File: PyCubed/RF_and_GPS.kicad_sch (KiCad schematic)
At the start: 45 parts, among them IC2 PCF8523T_1,118, J11 73412-0114, J12 73412-0114, J7 73412-0114, Q17 BSS138DWQ-7, Q28 MBT2222ADW1T1, Q29 BSS138DWQ-7, Q30 MBT2222ADW1T1, U10 XTB-40, U12 XTB-40, U13 EP2W+, U14 S1216V8, U20 RFM9xBreakout, U23 RFM98PW

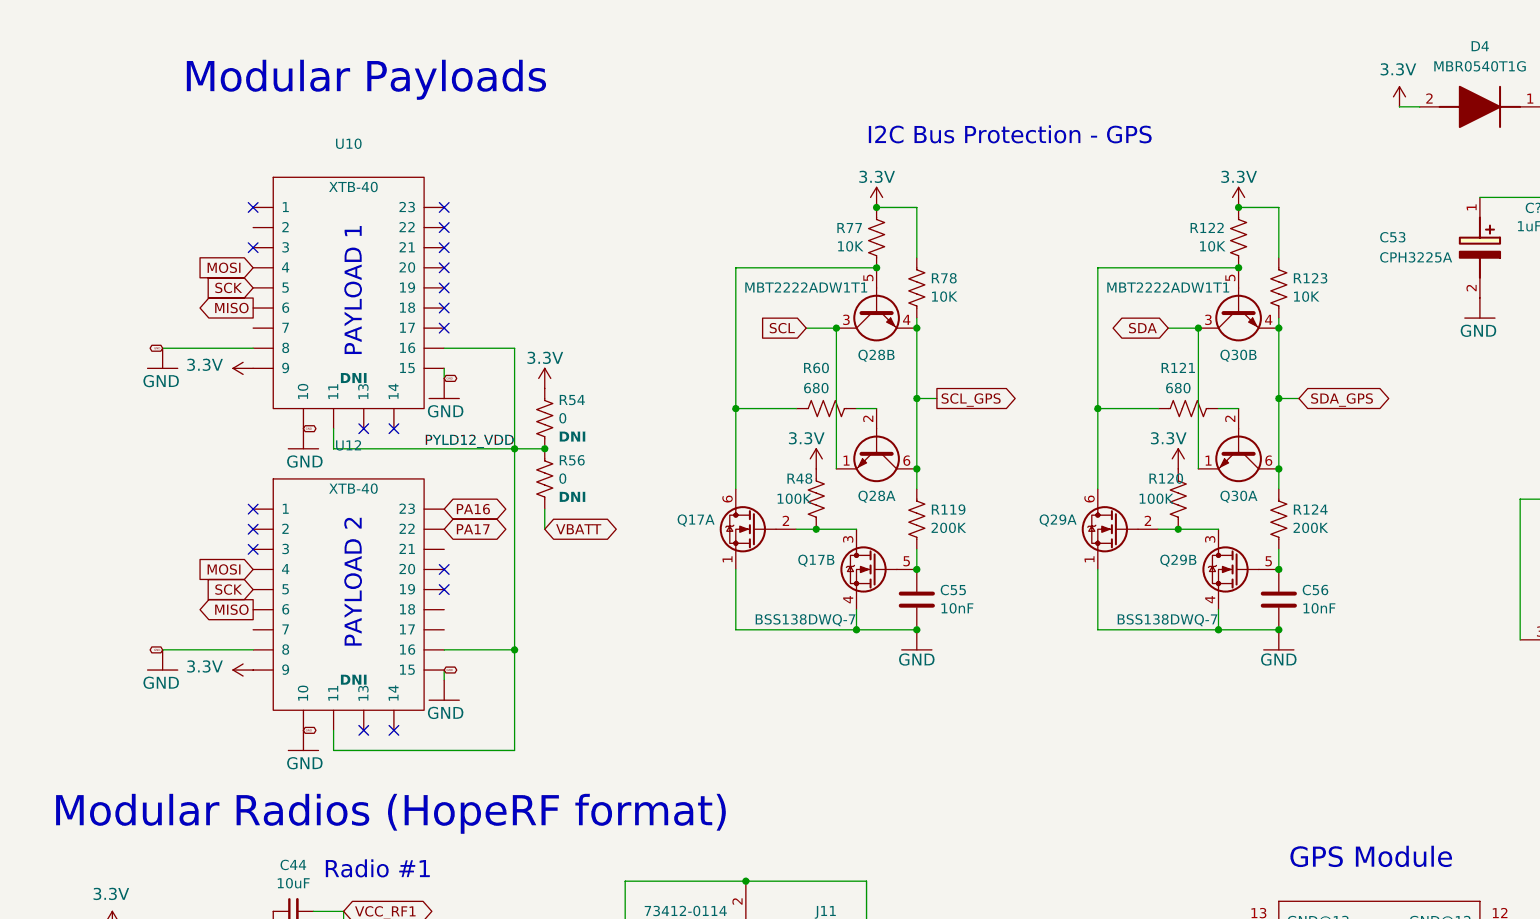
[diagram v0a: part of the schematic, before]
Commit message: PyCubed Routing Done
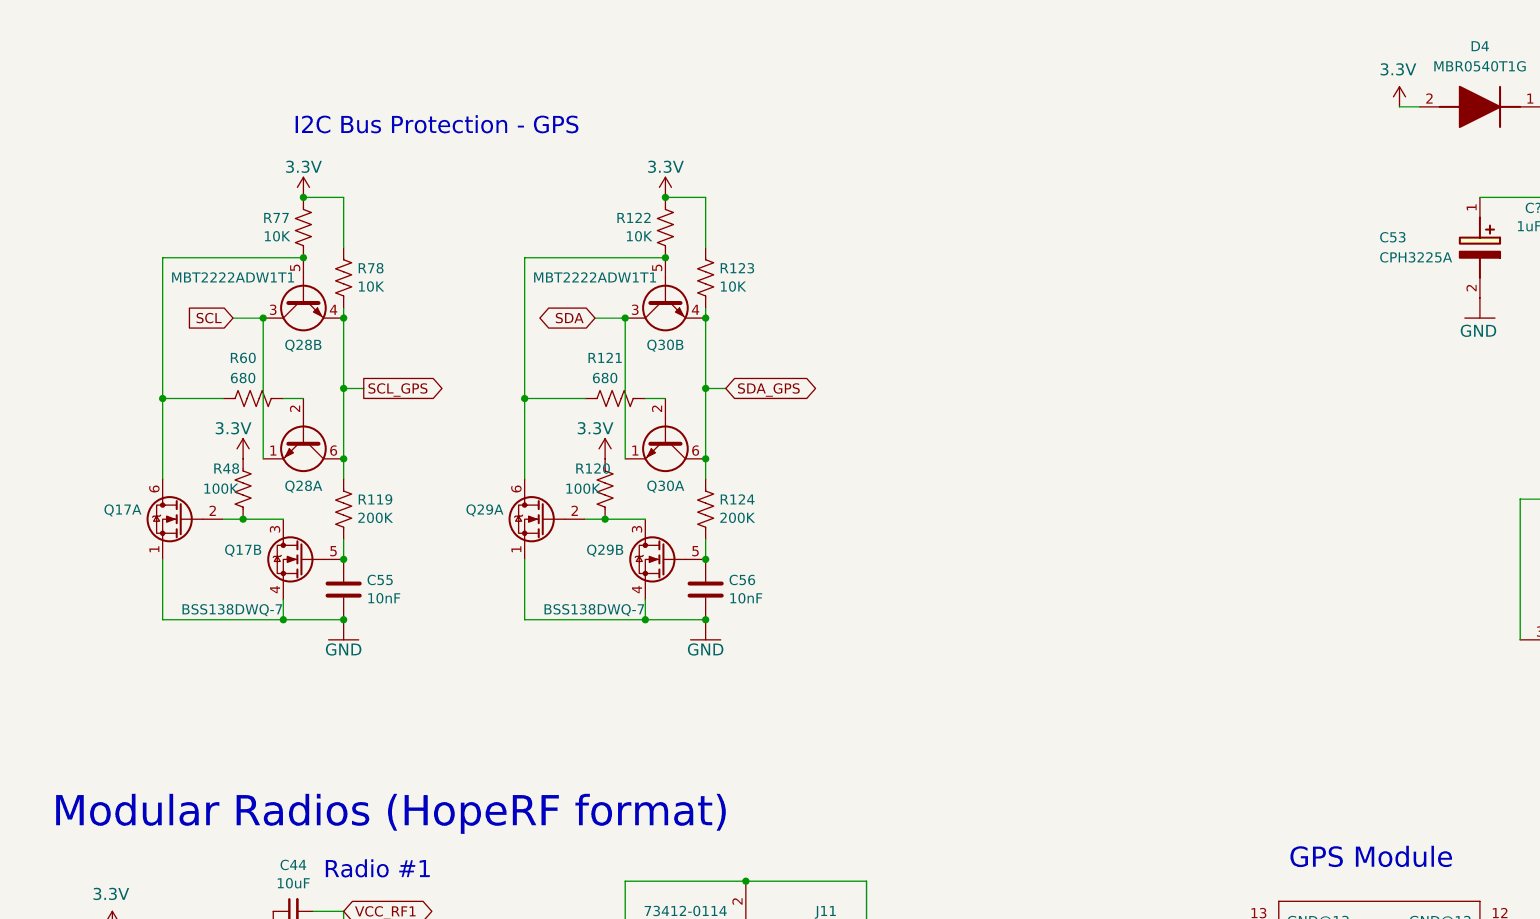
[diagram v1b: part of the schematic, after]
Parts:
- removed R54, R56: 0, Resistor_SMD:R_0805_2012Metric, symbol Device:R_US
- removed U10, U12: XTB-40, mainboard:XTB40_payload, symbol mainboard:XTB-40_payload
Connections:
- no-connect marks 40 -> 22
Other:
- note removed: "Modular Payloads"
- note removed: "PAYLOAD 1"
- note removed: "PAYLOAD 2"
- moved on the sheet: C55, C56, Q17A, Q17B, Q28A, Q28B, Q29A, Q29B, Q30A, Q30B, R119, R120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
